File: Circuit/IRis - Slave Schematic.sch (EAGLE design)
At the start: 15 parts, among them U1 ATTINY85SU

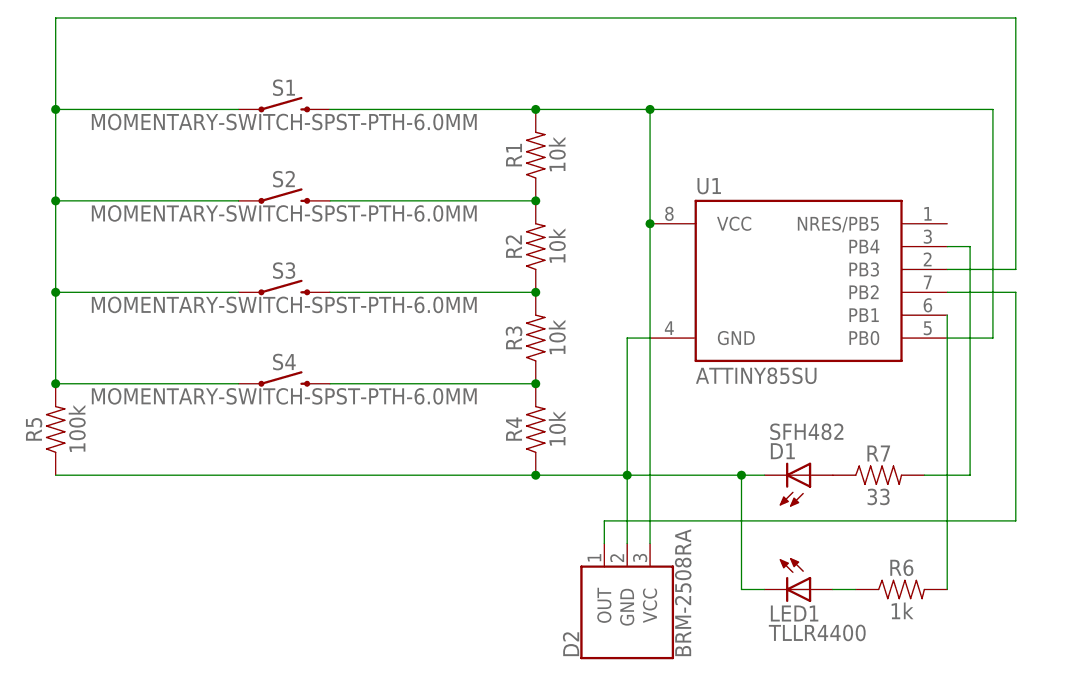
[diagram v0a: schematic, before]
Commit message: PCB Layout Added
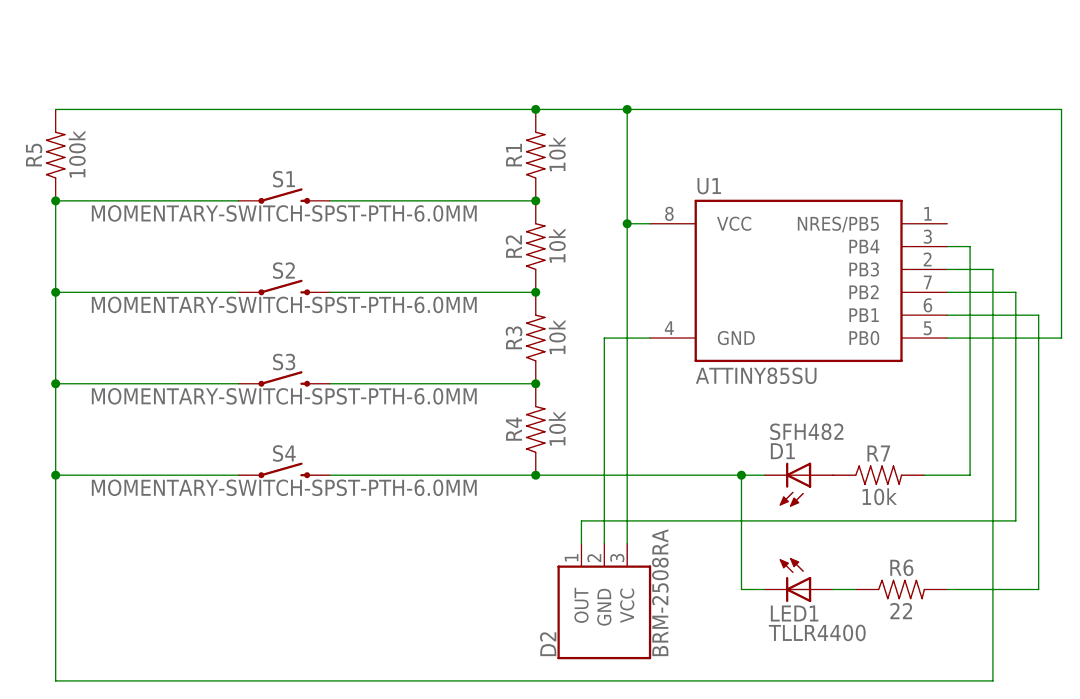
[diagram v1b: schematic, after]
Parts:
- R6: value 1k -> 22
- R7: value 33 -> 10k
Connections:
- removed net N$6: D1.C, D2.GND, LED1.C, R4.1, R5.1, U1.GND
- new net N$10: D2.VCC, R1.2, R5.2, U1.PB0, U1.VCC
- new net N$12: R1.1, R2.2, S1.2
- net N$1: now also R2.1, R3.2; no longer R1.1, R2.2
- net N$2: now also R3.1, R4.2; no longer R2.1, R3.2
- net N$3: now also D1.C, LED1.C, R4.1; no longer R3.1, R4.2
- net N$4: now also D2.GND, U1.GND; no longer D2.VCC, R1.2, S1.2, U1.PB0, U1.VCC
- net N$5: now also R5.1; no longer R5.2
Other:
- moved on the sheet: D2, R5, S1, S2, S3, S4
